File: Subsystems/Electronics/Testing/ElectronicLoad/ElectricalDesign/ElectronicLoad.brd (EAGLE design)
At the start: 104 x 130 mm, 85 parts, among them J1 USB, J2 Load, J3 Alternate Current Sense, J4 Voltage Sense, J5 SWD, J6 FAN, J7 12 V Input, Q1 IRFP4368PBF, Q2 SiRA20DP, Q3 SiRA20DP, Q4 IRFP4368PBF, SW1 Nice Knob, SW2 Nice Button, U1 STM32L476RGT, U2 AD8515, U3 FT230XQ, U4 INA199C1, U5 LP5907MFX-3.1, U6 INA199C1, Y1 8MHz ±10ppm

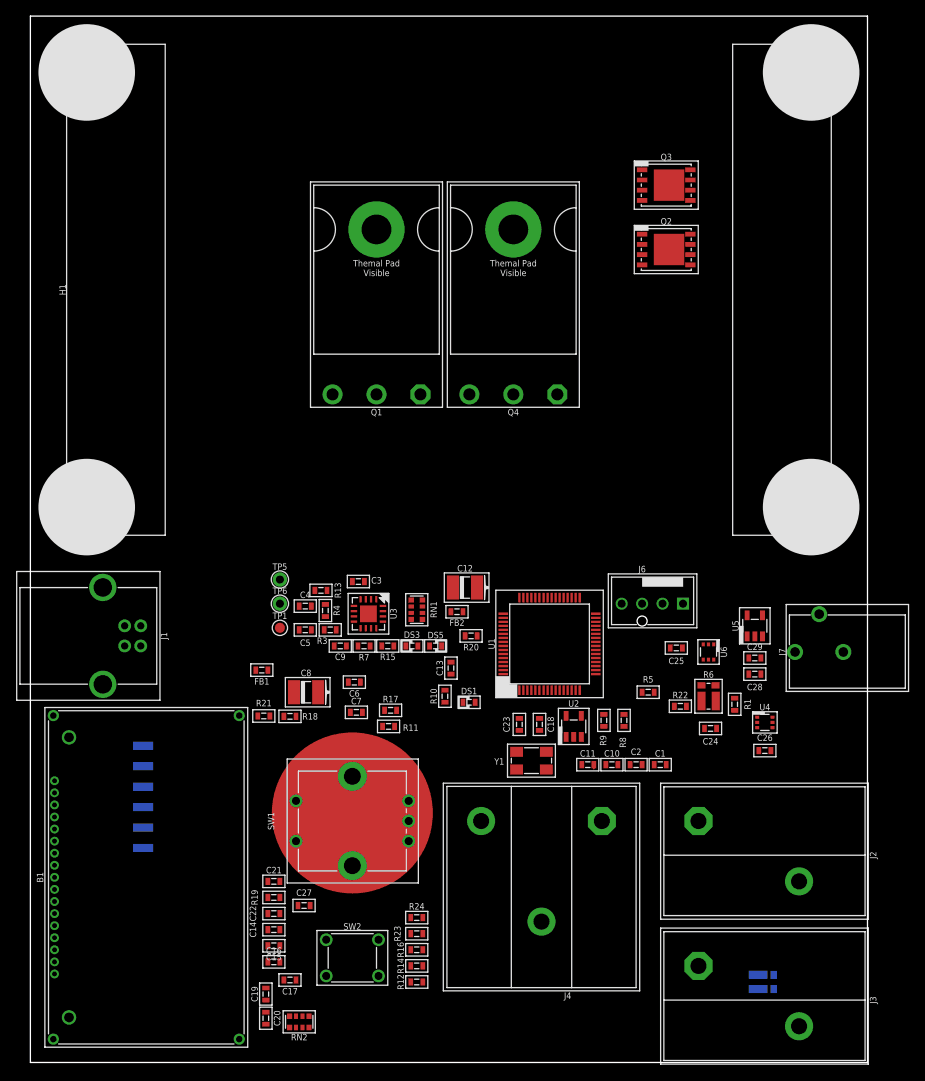
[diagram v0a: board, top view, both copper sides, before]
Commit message: worked on layout
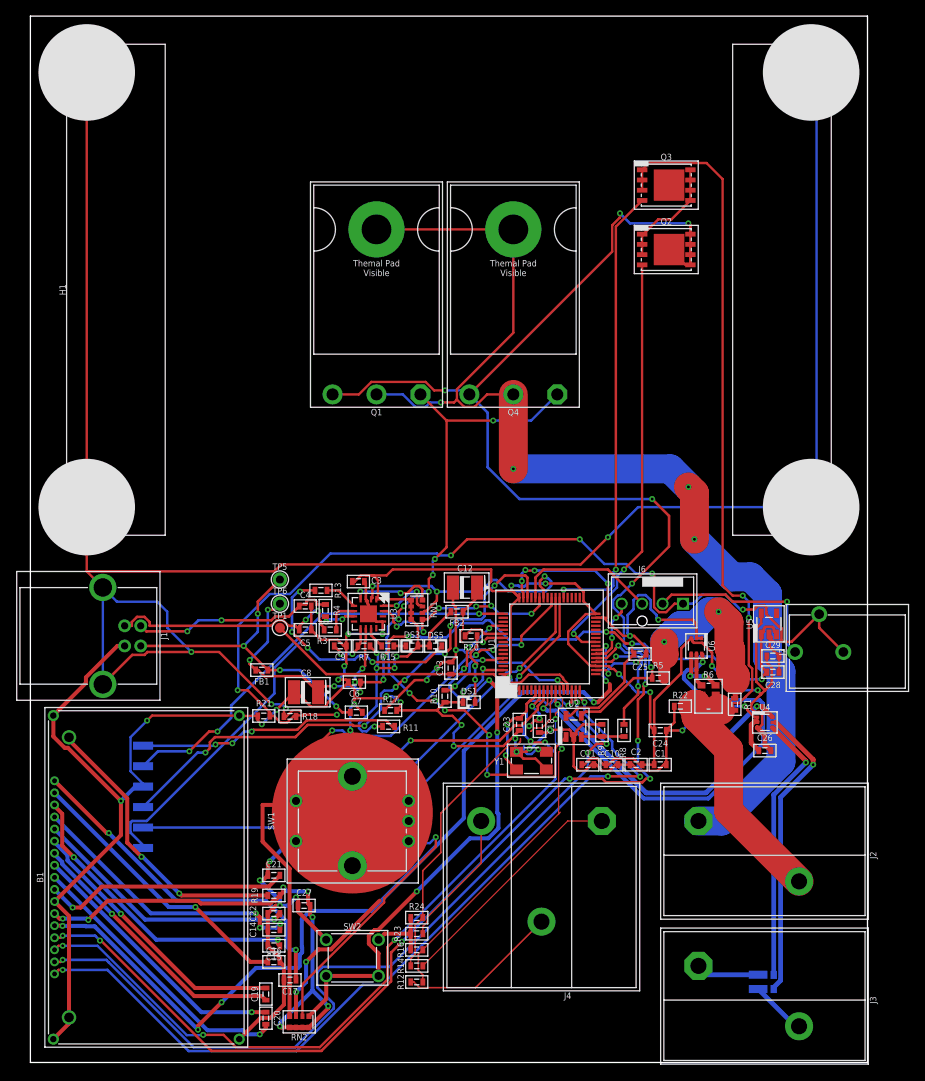
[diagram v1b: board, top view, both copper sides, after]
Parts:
- moved C24 6.25 mm to (26.2, -23.8)
- moved C25 4.56 mm to (23.8, -14.2)
- moved C28 2.26 mm to (40.2, -16.5)
- moved C29 2.26 mm to (40.2, -14.5)
- moved R5 2.15 mm to (26.0, -17.2)
- moved U5 1.77 mm to (39.8, -10.5)
- moved U6 1.68 mm to (30.8, -13.2)
- moved R9 1.27 mm to (19.0, -23.8)
- moved R8 1.25 mm to (21.8, -23.8)
- moved C21 0.75 mm to (-21.8, -41.8)
- moved C18 0.25 mm to (11.2, -23.2)
- moved R19 0.25 mm to (-21.8, -44.2)
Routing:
- net CHASSIS: track 0.00 -> 517.8 mm, vias 0 -> 4
- net DGND: track 0.50 -> 382.7 mm, vias 0 -> 35
- net 3.1V: track 0.00 -> 250.8 mm, vias 0 -> 20
- net LOAD_INPUT+: track 0.00 -> 146.8 mm, vias 0 -> 4
- net FEEDBACK: track 0.00 -> 145.9 mm, vias 0 -> 6
- net PGND: track 0.00 -> 125.4 mm, vias 0 -> 6
- net SPI_SCK: track 0.00 -> 120.0 mm, vias 0 -> 8
- net 5.0V: track 0.00 -> 118.0 mm, vias 0 -> 12
- net SPI_MOSI: track 0.00 -> 108.9 mm, vias 0 -> 6
- net !LCD_CS: track 0.00 -> 105.1 mm, vias 0 -> 4
- net LCD_A0: track 0.00 -> 104.2 mm, vias 0 -> 6
- net !LCD_RST: track 0.00 -> 103.8 mm, vias 0 -> 4
- net FET_GATE: track 0.00 -> 89.9 mm, vias 0 -> 11
- net SHUNT_LOW: track 0.00 -> 86.7 mm, vias 0 -> 2
- net ENC_SW: track 0.00 -> 78.8 mm, vias 0 -> 5
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
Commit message: Board Layout finished
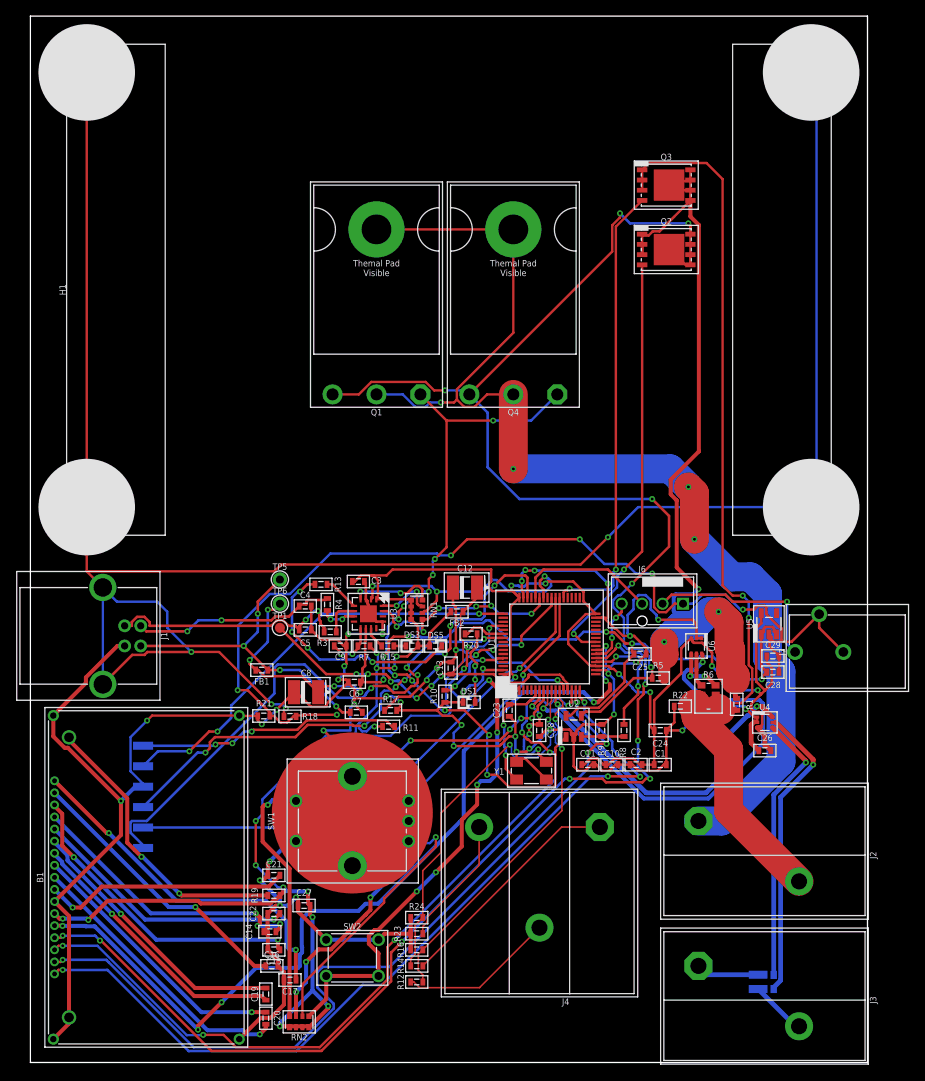
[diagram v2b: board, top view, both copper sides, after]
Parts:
- moved C23 2.15 mm to (7.50, -21.2)
- moved Y1 1.25 mm to (10.2, -28.8)
- moved J4 0.79 mm to (18.8, -35.8)
- moved R4 0.79 mm to (-15.1, -8.10)
- moved R13 0.75 mm to (-15.9, -5.60)
- moved C14 0.56 mm to (-22.2, -48.8)
- moved C16 0.56 mm to (-22.0, -53.0)
- moved C15 0.50 mm to (-21.8, -51.0)
- moved C18 0.50 mm to (11.2, -23.8)
- moved R1 0.25 mm to (35.8, -20.5)
- moved R20 0.25 mm to (2.75, -11.8)
- moved R3 0.25 mm to (-14.8, -11.5)
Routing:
- net SHUNT_MID: track 42.5 -> 111.8 mm, vias 2 -> 3
- net DGND: track 382.7 -> 415.5 mm
- net 3.1V: track 250.8 -> 281.7 mm, vias 20 -> 22
- net SWO: track 38.8 -> 69.1 mm, vias 1 -> 4
- net ENC_B: track 53.0 -> 66.9 mm, vias 3 -> 4
- net CHASSIS: track 517.8 -> 531.6 mm
- net AVDD: track 48.2 -> 55.8 mm, vias 0 -> 6
- net V_ALT: track 41.2 -> 47.2 mm, vias 0 -> 2
- net FEEDBACK: track 145.9 -> 140.7 mm
- net OSC_OUT: track 9.76 -> 13.9 mm, vias 4 -> 5
- net LOAD_INPUT-: track 30.0 -> 34.0 mm
- net SHUNT_LOW: track 86.7 -> 90.2 mm
- net OSC_IN: track 12.4 -> 14.7 mm
- net FET_GATE: track 89.9 -> 91.7 mm
- net I_LOAD: track 59.3 -> 58.0 mm
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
